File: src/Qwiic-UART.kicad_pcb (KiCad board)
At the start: 2 copper layers, 25.4 x 25.4 mm, 16 parts, among them J1 QWIIC, J2 QWIIC, J3 FTDI, U1 SC16IS740, X1 ECS-2520MVLC-018-BN-TR

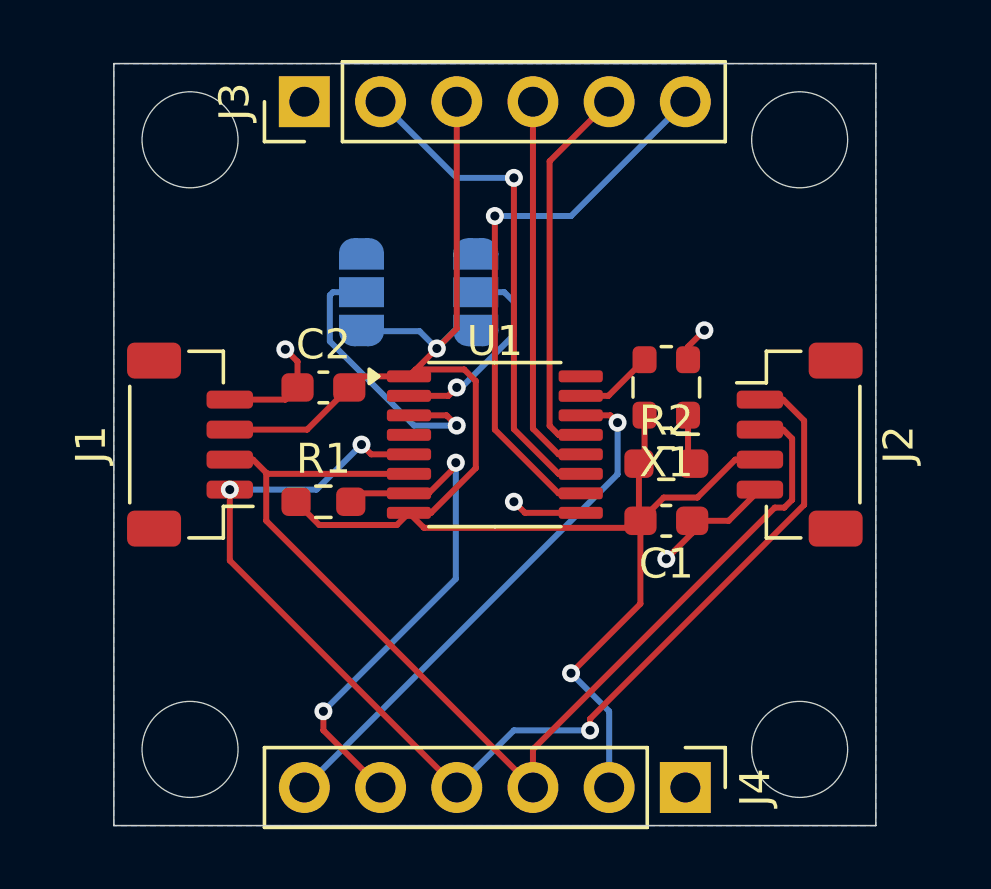
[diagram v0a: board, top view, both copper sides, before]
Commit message: Made some refinements
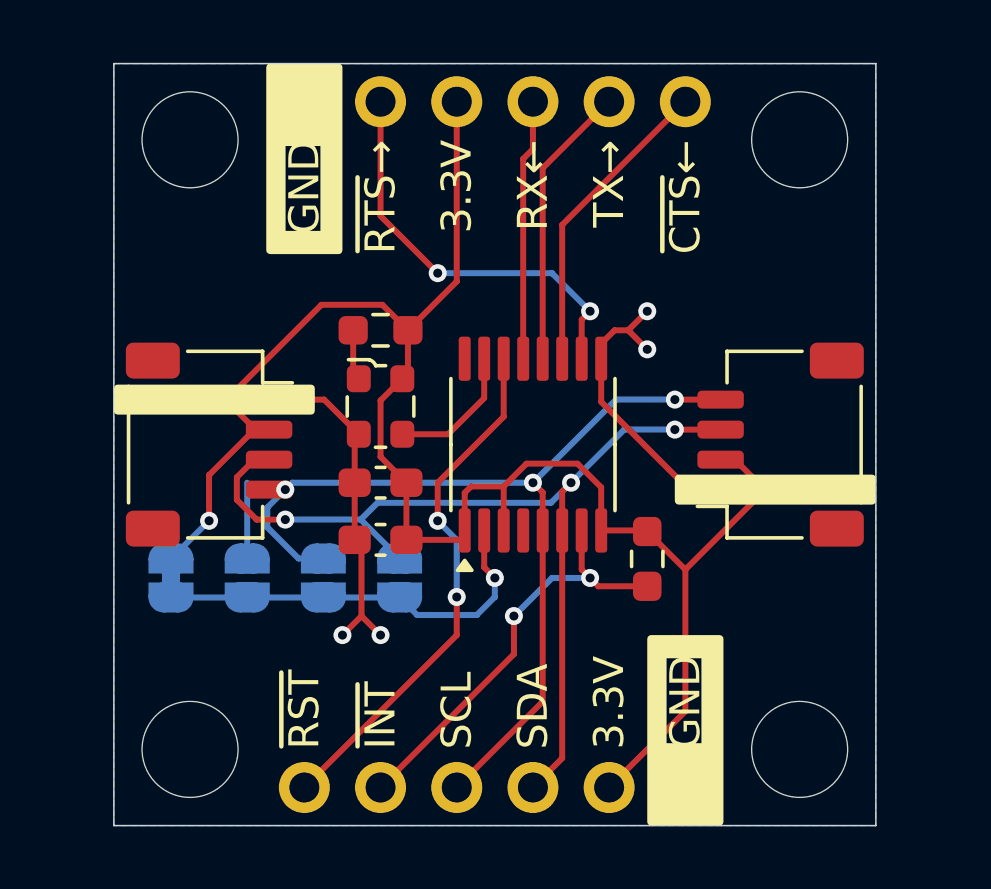
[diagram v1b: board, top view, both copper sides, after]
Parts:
- added JP3: SolderJumper_2_Open, Jumper:SolderJumper-2_P1.3mm_Open_RoundedPad1.0x1.5mm, B.Cu at (134.0, 112.4)
- added JP4: SolderJumper_2_Open, Jumper:SolderJumper-2_P1.3mm_Open_RoundedPad1.0x1.5mm, B.Cu at (136.5, 112.4)
- J1, J2: footprint Connector_JST:JST_SH_BM04B-SRSS-TB_1x04-1MP_P1.00mm_Vertical -> Connector_JST:JST_SH_SM04B-SRSS-TB_1x04-1MP_P1.00mm_Horizontal
- J3, J4: footprint Connector_PinHeader_2.54mm:PinHeader_1x06_P2.54mm_Vertical -> Project_Footprints:PinHeader_1x06_P2.54mm
- JP1: value SolderJumper_3_Open -> SolderJumper_2_Bridged; footprint Jumper:SolderJumper-3_P1.3mm_Open_RoundedPad1.0x1.5mm -> Jumper:SolderJumper-2_P1.3mm_Bridged_RoundedPad1.0x1.5mm
- JP2: value SolderJumper_3_Open -> SolderJumper_2_Open; footprint Jumper:SolderJumper-3_P1.3mm_Open_RoundedPad1.0x1.5mm -> Jumper:SolderJumper-2_P1.3mm_Open_RoundedPad1.0x1.5mm
- REF** (x4): value MountingHole_3.2mm_M3 -> MountingHole_3.2mm; footprint MountingHole:MountingHole_3.2mm_M3 -> Project_Footprints:MountingHole_3.2mm
- moved JP1 13.9 mm to (128.9, 112.4)
- moved R1 11.0 mm to (144.8, 111.8), turned to -90 degrees
- moved R2 10.5 mm to (135.9, 104.1), turned to 180 degrees
- moved JP2 10.3 mm to (131.4, 112.4)
- moved C1 9.61 mm to (135.9, 109.2), turned to 0 degrees
- moved X1 9.55 mm to (135.9, 106.7), turned to 0 degrees
- moved C2 5.43 mm to (135.9, 111.1)
- moved U1 1.27 mm to (141.0, 108.0), turned to 90 degrees
- moved J1 0.64 mm to (130.2, 108.0), turned to -90 degrees
- moved J2 0.64 mm to (149.2, 108.0), turned to 90 degrees
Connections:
- J1 pad 1: /SCL -> GND
- J1 pad 2: /SDA -> +3.3V
- J1 pad 3: +3.3V -> /SDA
- J1 pad 4: GND -> /SCL
- J2 pad 1: /SCL -> GND
- J2 pad 2: /SDA -> +3.3V
- J2 pad 3: +3.3V -> /SDA
- J2 pad 4: GND -> /SCL
- J3 pad 2: /~{CTS} -> /~{RTS}
- J3 pad 4: /TX -> /RX
- J3 pad 5: /RX -> /TX
- J3 pad 6: /~{RTS} -> /~{CTS}
- JP1 pad 1: GND -> +3.3V
- JP2 pad 2: /A1 -> /A0
- U1 pad 3: /A1 -> +3.3V
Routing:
- net GND: track 11.8 -> 24.0 mm
- net /A1: track 9.76 -> 0.00 mm, vias 1 -> 0
- net /SCL: track 40.1 -> 31.6 mm
- net /A0: track 6.85 -> 13.7 mm
- net /~{CTS}: track 16.7 -> 10.3 mm, vias 1 -> 0
- net /~{RTS}: track 18.8 -> 13.8 mm, vias 1 -> 2
- net /SDA: track 36.9 -> 32.2 mm, vias 0 -> 3
- net /RX: track 12.8 -> 8.70 mm
- net /TX: track 12.8 -> 9.48 mm
- net /~{INT}: track 17.6 -> 14.3 mm
- net /CLK: track 2.63 -> 4.54 mm
- net /~{RST}: track 17.8 -> 17.6 mm, vias 1 -> 2
- net +3.3V: track 60.1 -> 59.9 mm, vias 2 -> 1
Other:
- board text added: "0x90"
- board text added: "0x92"
- board text added: "0x94"
- board text added: "0x96"
- board text added: "3.3V"
- board text added: "GND"
- board text added: "QWIIC"
- board text added: "REV: 0.0.1"
- board text added: "RX←"
- board text added: "SCL"
- board text added: "SDA"
- board text added: "TX→"
- board text added: "UART"
- board text added: "~{CTS}←"
- board text added: "~{INT}"
- board text added: "~{RST}"
- board text added: "~{RTS}→"
